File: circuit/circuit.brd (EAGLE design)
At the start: 41.6 x 34.3 mm, 16 parts, among them IC1 AT90S2313P, Q1 16MHz

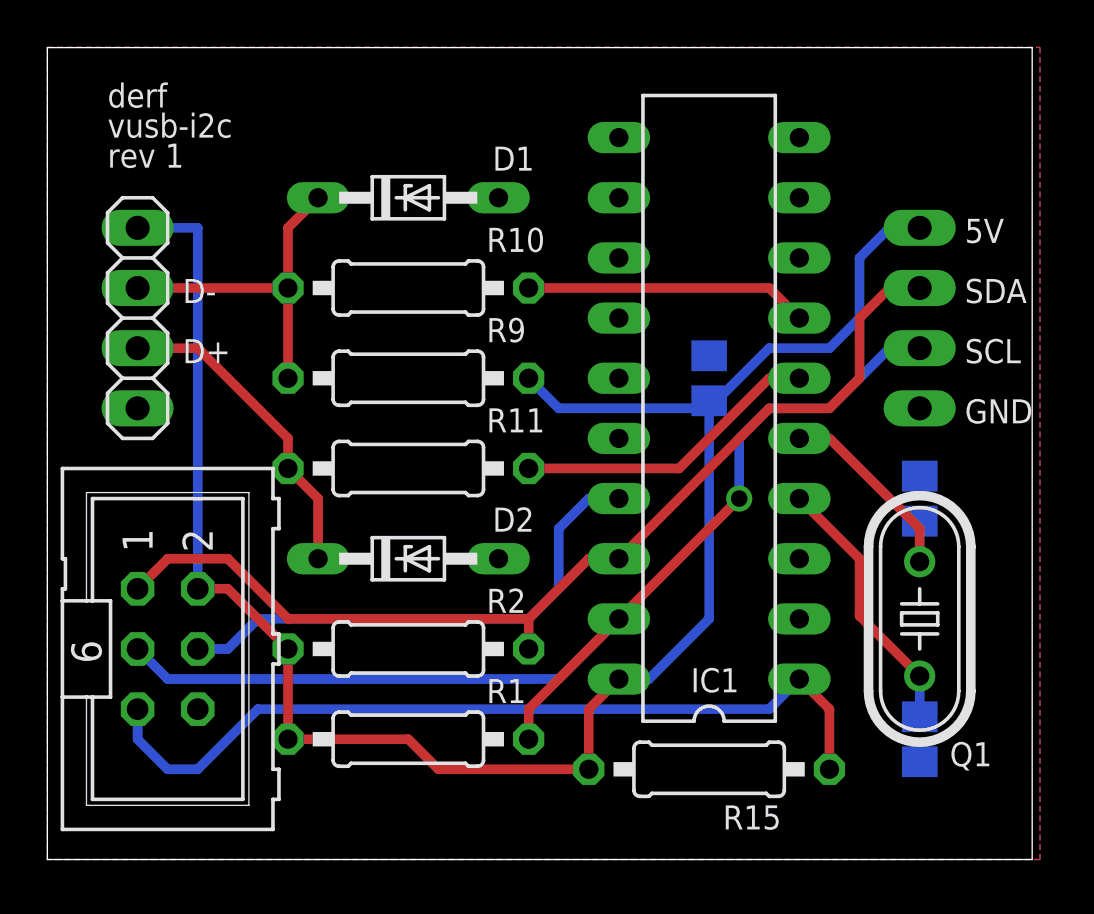
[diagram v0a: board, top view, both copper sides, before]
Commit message: more layouting
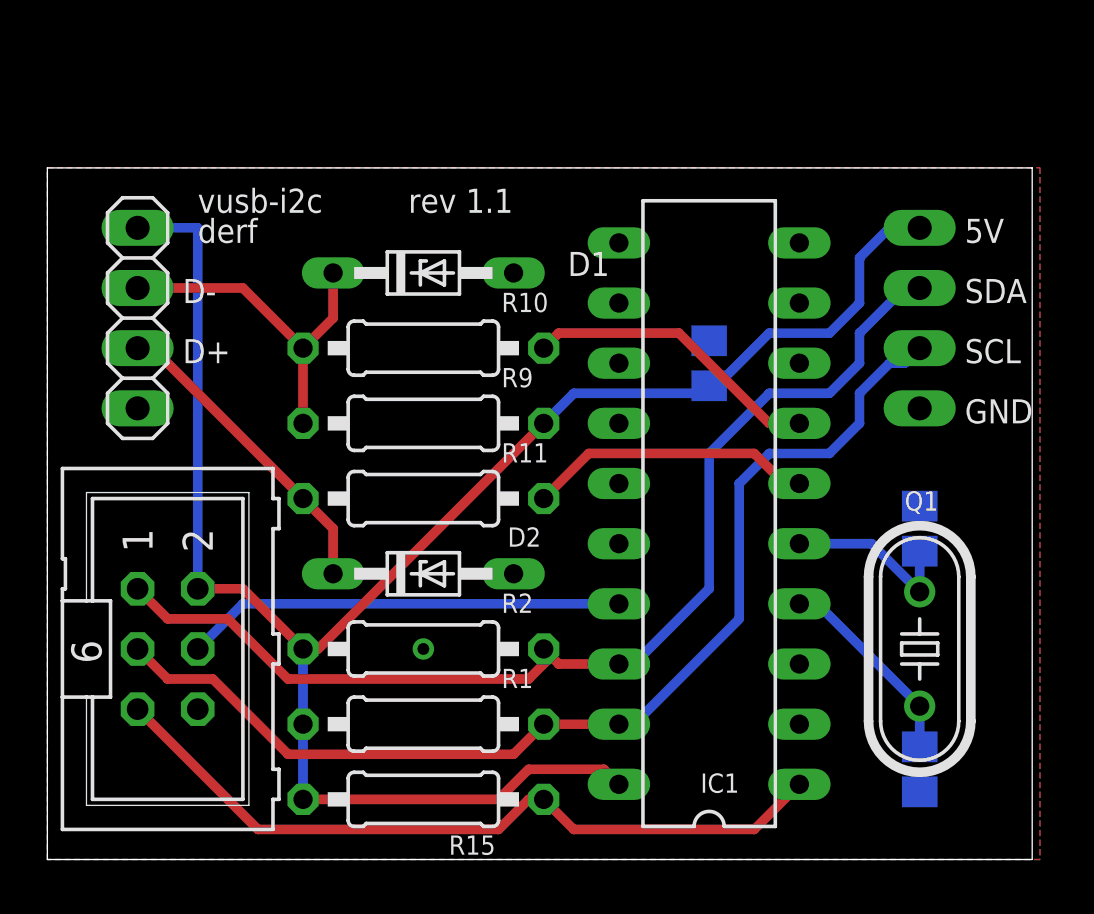
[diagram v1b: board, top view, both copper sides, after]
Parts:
- moved R15 12.1 mm to (15.9, 2.54)
- moved IC1 4.45 mm to (27.9, 14.6)
- moved D1 3.24 mm to (15.9, 24.8)
- moved R10 2.62 mm to (15.9, 21.6)
- moved R9 2.01 mm to (15.9, 18.4)
- moved R11 1.42 mm to (15.9, 15.2)
- moved C5 1.27 mm to (36.8, 3.81)
- moved C4 1.27 mm to (36.8, 14.0)
- moved Q1 1.27 mm to (36.8, 8.89)
- moved D2 0.90 mm to (15.9, 12.1)
- moved R1 0.90 mm to (15.9, 5.71)
- moved R2 0.63 mm to (15.9, 8.89)
- moved C6 0.63 mm to (27.9, 21.0)
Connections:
- net N$27 renamed AVRD+
- net N$41 renamed AVRD-
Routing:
- net N$1: track 35.7 -> 31.9 mm
- net N$4: track 21.9 -> 18.6 mm
- net SDA: track 43.1 -> 46.2 mm
- net N$38: track 11.3 -> 8.59 mm
- net N$37: track 9.77 -> 7.64 mm
- net SCL: track 47.5 -> 46.1 mm, vias 1 -> 0
- net VCC: track 79.6 -> 78.3 mm
- net AVRD+: track 13.0 -> 12.1 mm
- net AVRD-: track 12.0 -> 12.6 mm
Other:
- board size 41.6 x 34.3 mm -> 41.6 x 29.2 mm
- board text added: "rev 1.1"
- board text removed: "rev 1"
